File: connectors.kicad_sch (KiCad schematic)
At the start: 7 parts, among them J2 217183-0001, J3 BM03B-SRSS-TB

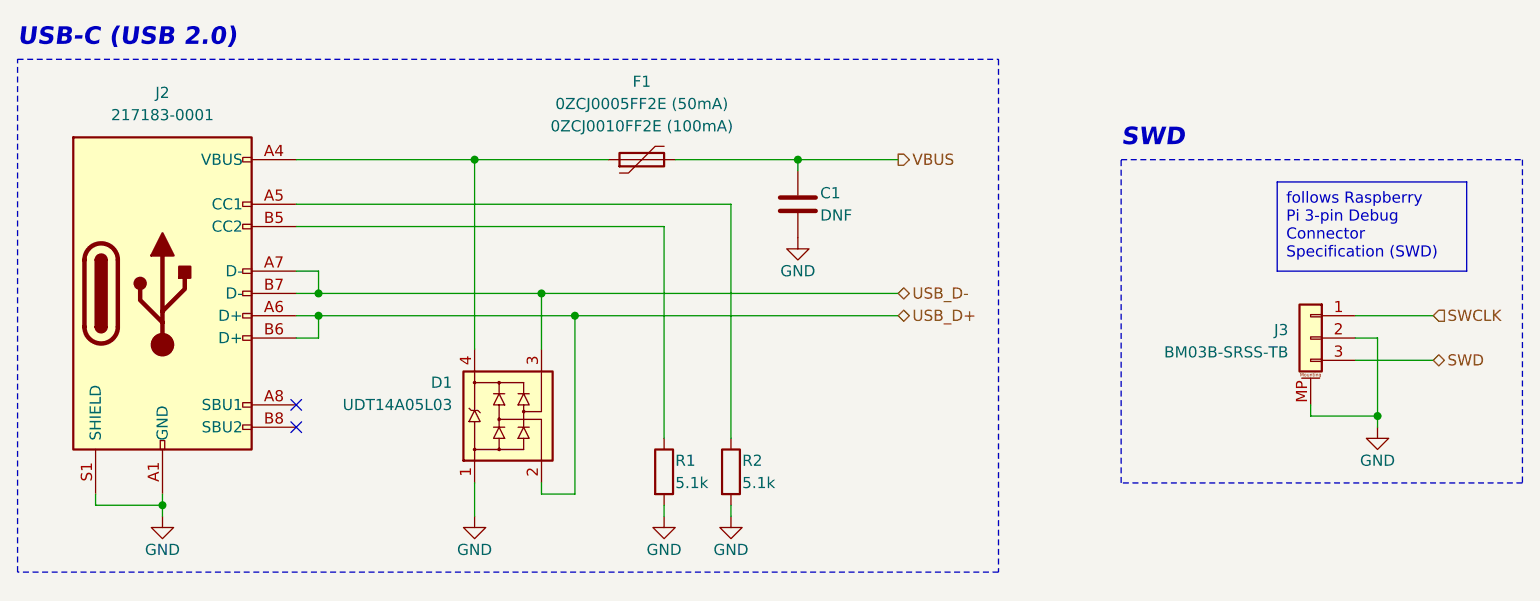
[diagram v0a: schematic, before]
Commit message: schematic cleanup
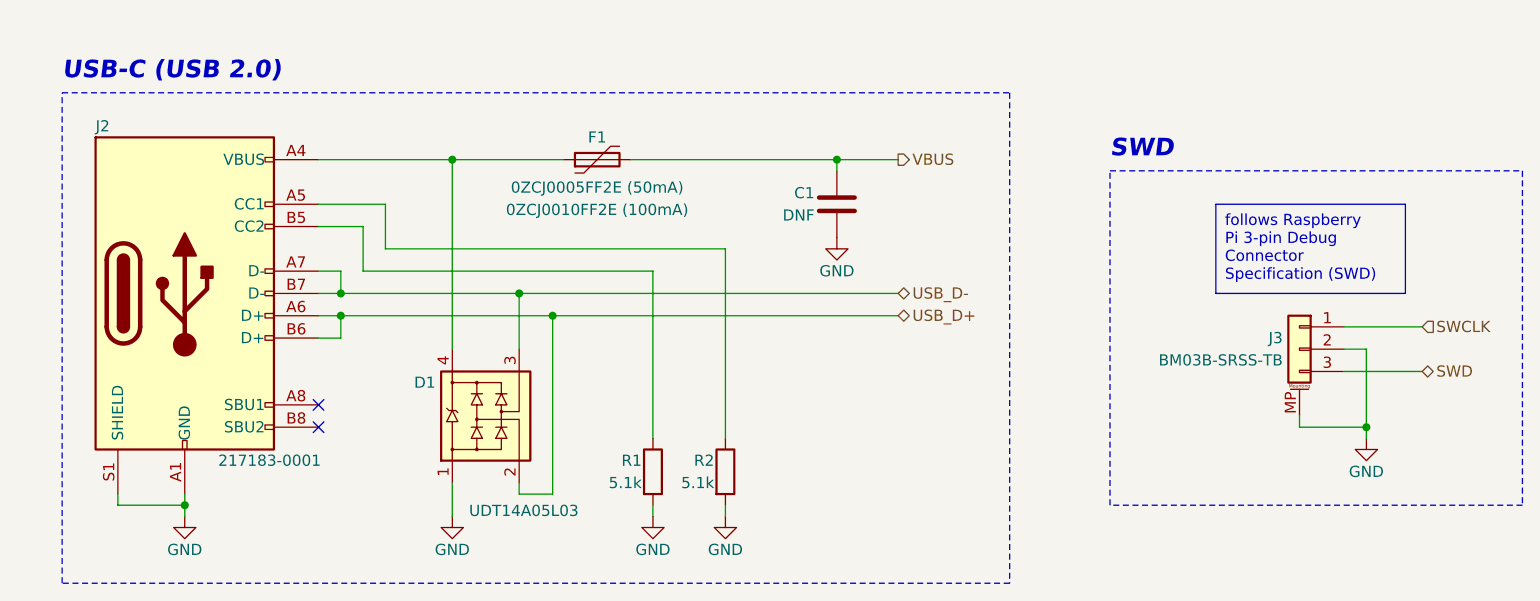
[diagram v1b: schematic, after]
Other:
- moved on the sheet: C1, D1, F1, J2, J3, R1, R2
